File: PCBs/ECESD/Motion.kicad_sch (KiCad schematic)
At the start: 11 parts, among them Q300 BSS138, Q301 BSS138, U300 ICM-20948

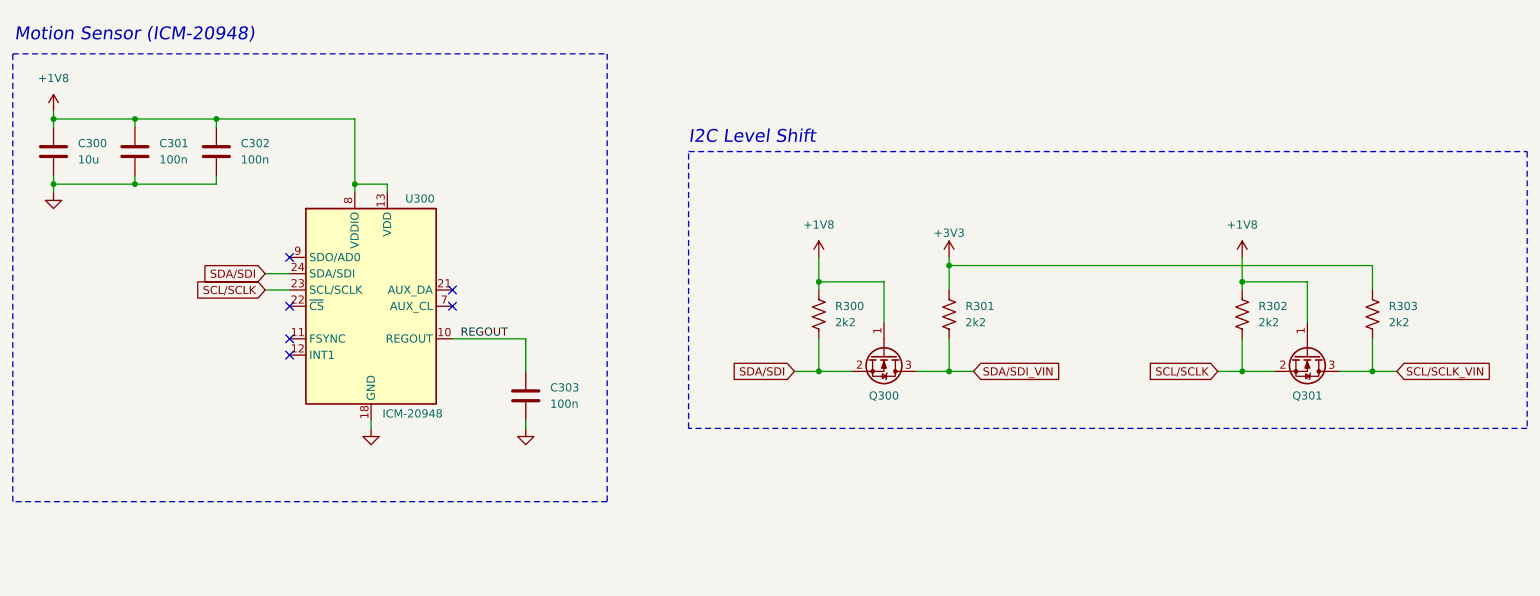
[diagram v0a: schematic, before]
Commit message: Changed PCB 1
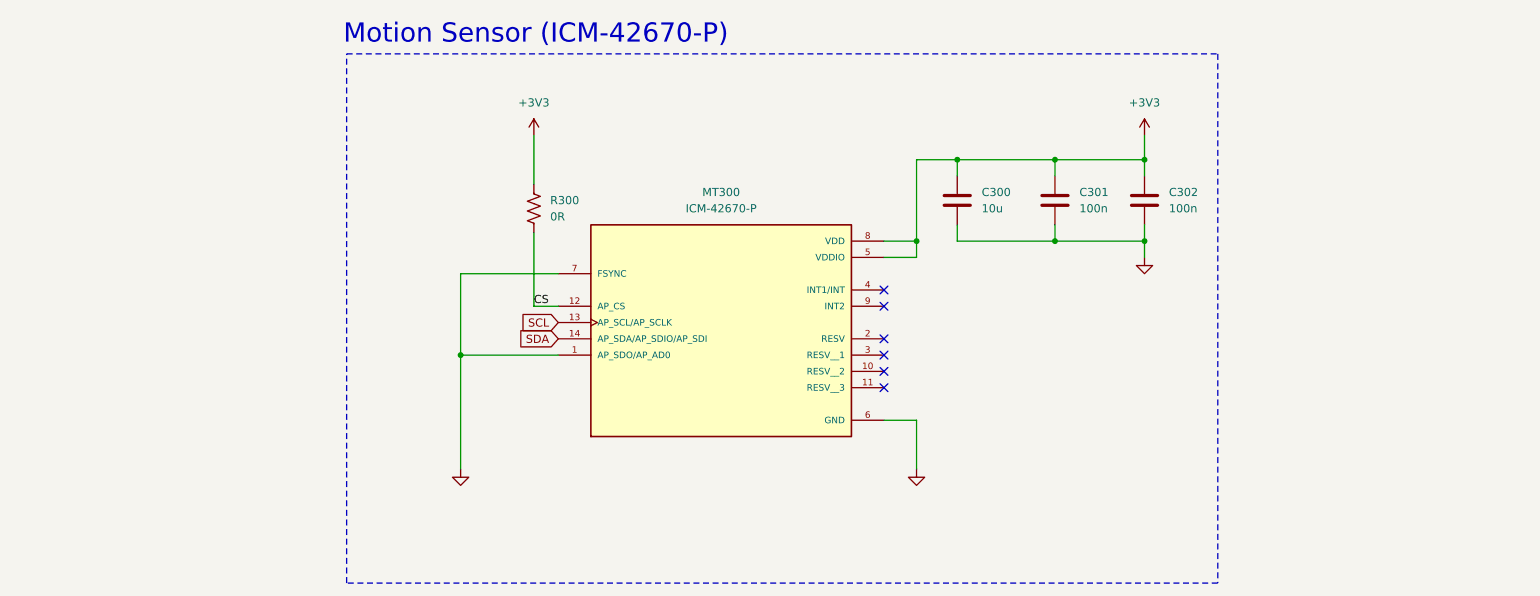
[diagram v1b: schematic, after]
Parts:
- removed C303: 100n, Capacitor_SMD:C_0603_1608Metric_Pad1.08x0.95mm_HandSolder, symbol Device:C
- removed Q300, Q301: BSS138, Package_TO_SOT_SMD:SOT-23, symbol Transistor_FET:BSS138
- removed R301, R302, R303: 2k2, Resistor_SMD:R_0603_1608Metric_Pad0.98x0.95mm_HandSolder, symbol Device:R_US
- removed U300: ICM-20948, Sensor_Motion:InvenSense_QFN-24_3x3mm_P0.4mm, symbol Sensor_Motion:ICM-20948
- added MT300: ICM-42670-P, ICM_42670_P:XDCR_ICM-42670-P, symbol ICM-42670-P:ICM-42670-P
- R300: value 2k2 -> 0R
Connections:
- net +1V8 is gone; now on net +3V3: C300.1, C301.1, C302.1, R300.1
- net +3V3: now also MT300.5 (VDDIO), MT300.8 (VDD)
- net GND: now also MT300.1 (AP_SDO/AP_AD0), MT300.6 (GND), MT300.7 (FSYNC)
- net SDA/SDI renamed CS
- net CS: now also MT300.12 (AP_CS)
- new net SCL: MT300.13 (AP_SCL/AP_SCLK)
- new net SDA: MT300.14 (AP_SDA/AP_SDIO/AP_SDI)
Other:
- note added: "Motion Sensor (ICM-42670-P)"
- note removed: "I2C Level Shift"
- note removed: "Motion Sensor (ICM-20948)"
